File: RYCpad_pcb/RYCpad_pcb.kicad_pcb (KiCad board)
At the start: 2 copper layers, 77.2 x 117.6 mm, 71 parts, among them J1 USB_C_Receptacle_USB2.0, J2 AVR ISP, K1 KEYSW, K10 KEYSW, K11 KEYSW, K12 KEYSW, K13 KEYSW, K14 KEYSW, K15 KEYSW, K16 KEYSW, K17 KEYSW, K2 KEYSW, K3 KEYSW, K4 KEYSW, K5 KEYSW, K6 KEYSW, K7 KEYSW, K8 KEYSW, K9 KEYSW, SW1 RESET, SW2 BOOT, U1 ATmega328P-PU, X1 16MHz

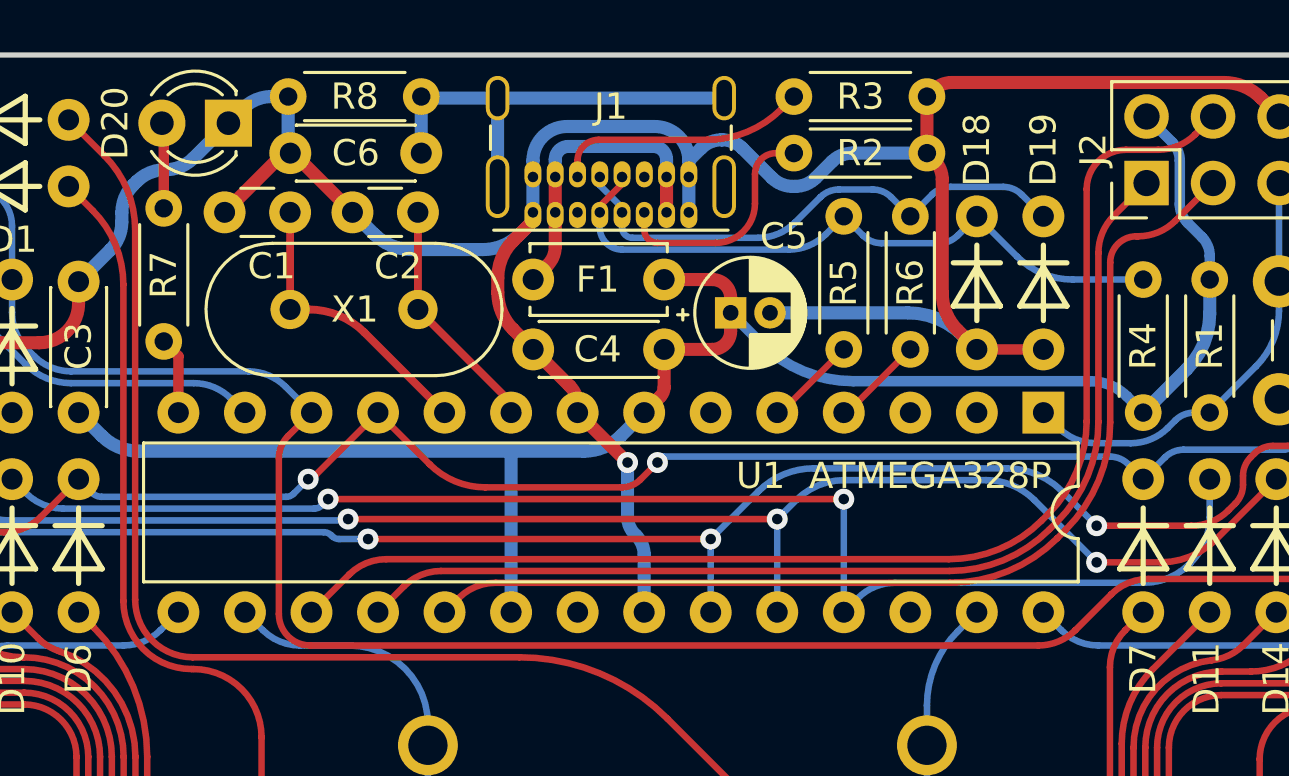
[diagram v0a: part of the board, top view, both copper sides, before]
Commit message: new render
- also, minor routing changes
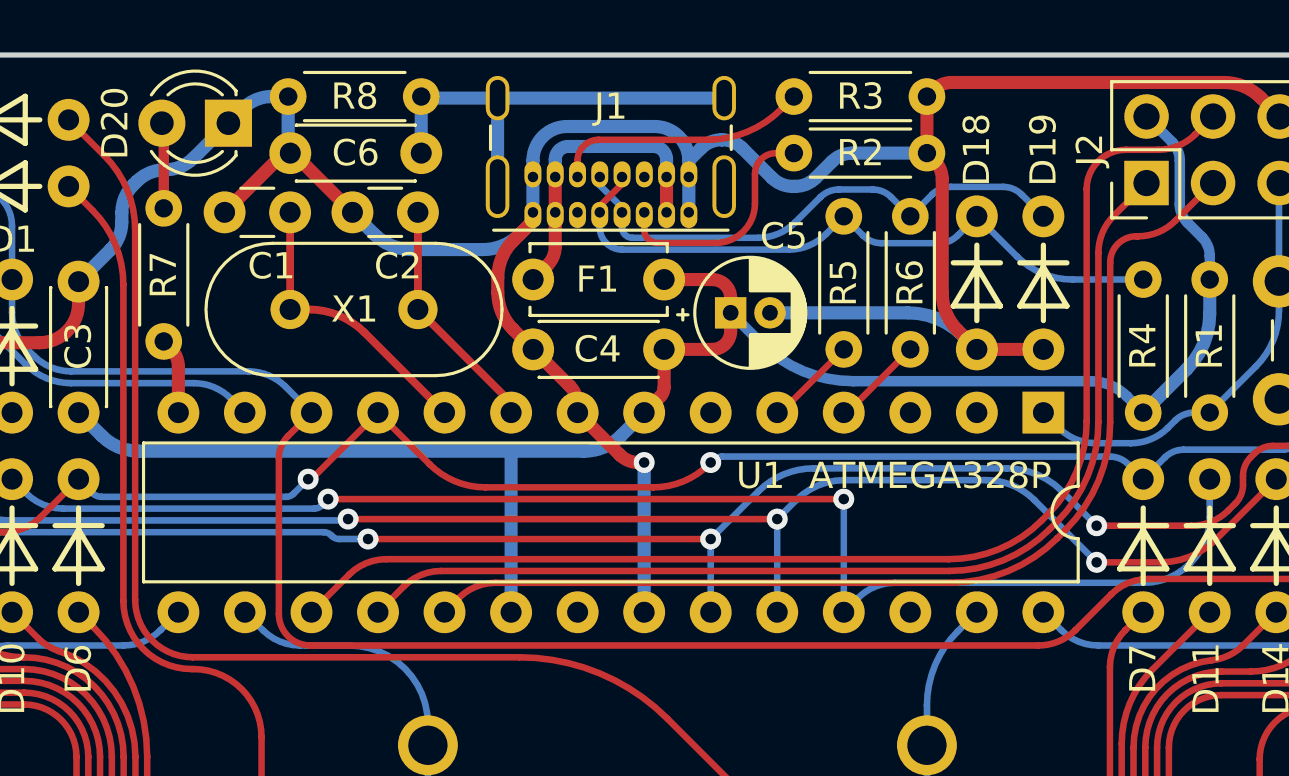
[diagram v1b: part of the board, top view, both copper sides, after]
